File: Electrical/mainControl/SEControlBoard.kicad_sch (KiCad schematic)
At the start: 56 parts, among them J10 BtottomButton, J11 Mouse1, J12 Mouse2, J14 USB_C_Receptacle_USB2.0_16P, J15 USB_A, J16 USB_A, J2 Encoder 1, J3 Encoder 2, J4 Conn_01x04, J5 Motor1, J6 Motor2, J7 Motor3, J8 Motor4, J9 TopButton, Q1 BSS138, Q2 BSS138, Q3 BSS138, Q4 BSS138, SW2 SW_MEC_5G, SW3 SW_MEC_5G, U1 BMI323, U2 AP63203WU, U3 ESP32-S3-MINI-1U, U4 TS3USB30EDGSR, U5 TS3USB30EDGSR

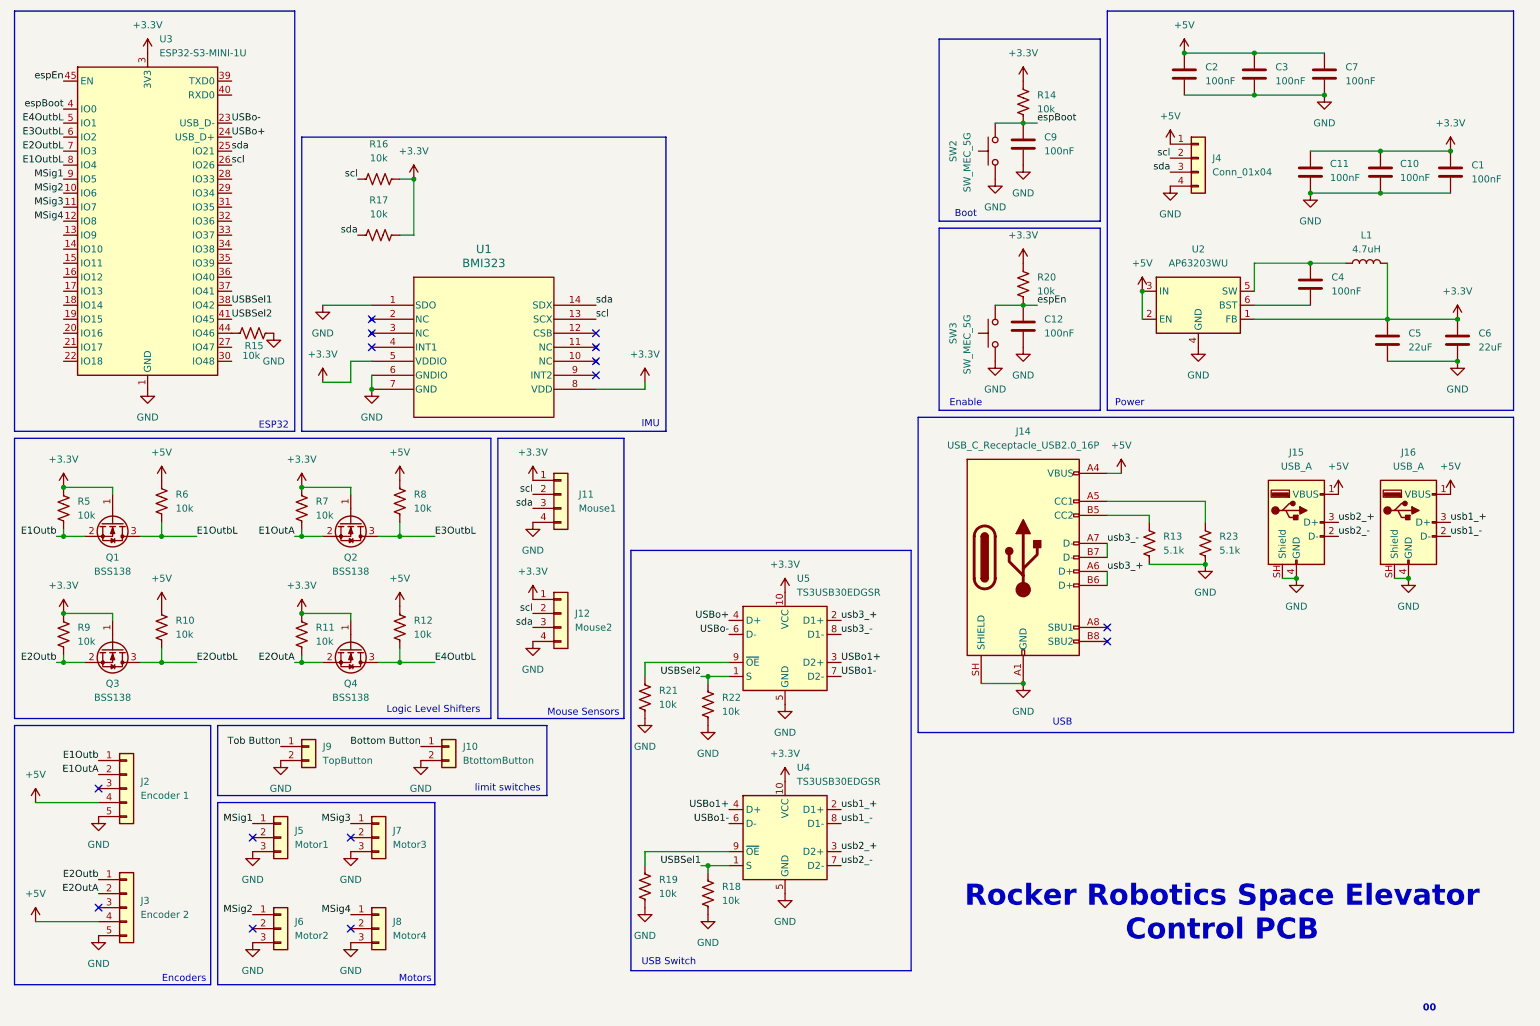
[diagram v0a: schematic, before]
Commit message: changed arrangment in schematic
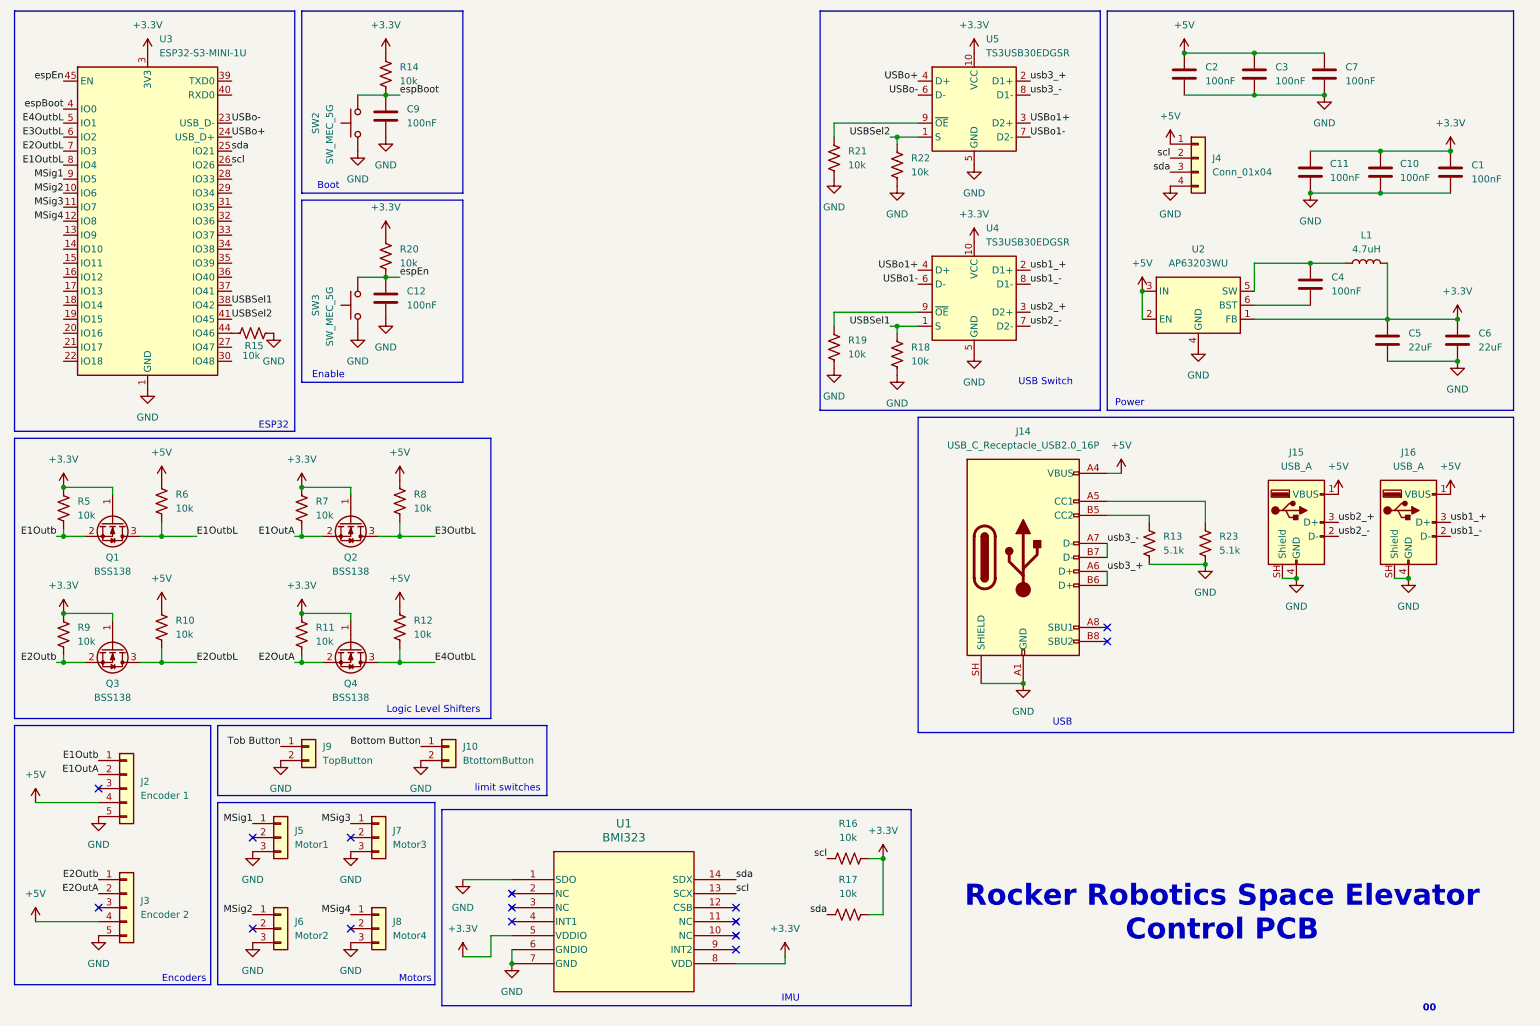
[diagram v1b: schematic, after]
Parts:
- removed J11: Mouse1, Connector_JST:JST_EH_B4B-EH-A_1x04_P2.50mm_Vertical, symbol Connector_Generic:Conn_01x04
- removed J12: Mouse2, Connector_JST:JST_EH_B4B-EH-A_1x04_P2.50mm_Vertical, symbol Connector_Generic:Conn_01x04
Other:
- note removed: "Mouse Sensors"
- moved on the sheet: C12, C9, R14, R16, R17, R18, R19, R20, R21, R22, SW2, SW3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
